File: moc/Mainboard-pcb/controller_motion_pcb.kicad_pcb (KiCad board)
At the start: 2 copper layers, 156 x 30 mm, 30 parts, among them J1 Conn_01x08_Female, J2 Conn_01x09_Male, J3 Conn_01x06_Female, SW1 Rotary_Encoder_Switch, U1 TPIC6C595-SOIC, U2 TPIC6C595-SOIC

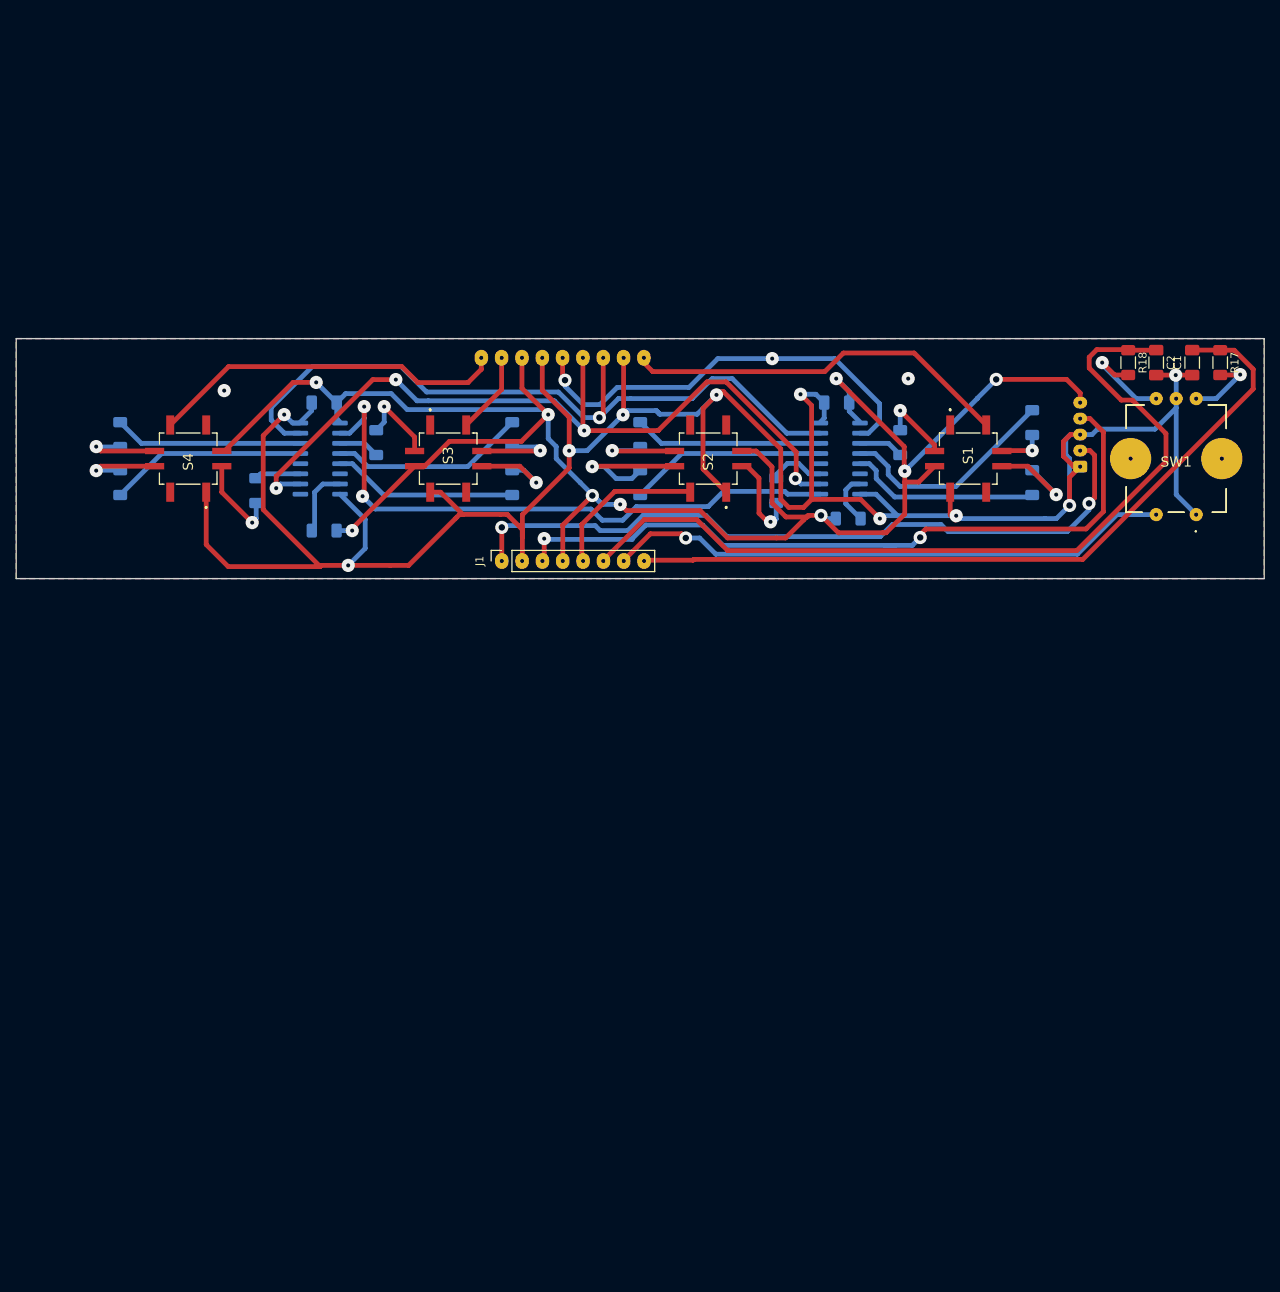
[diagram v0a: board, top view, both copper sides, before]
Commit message: hardware io funzt
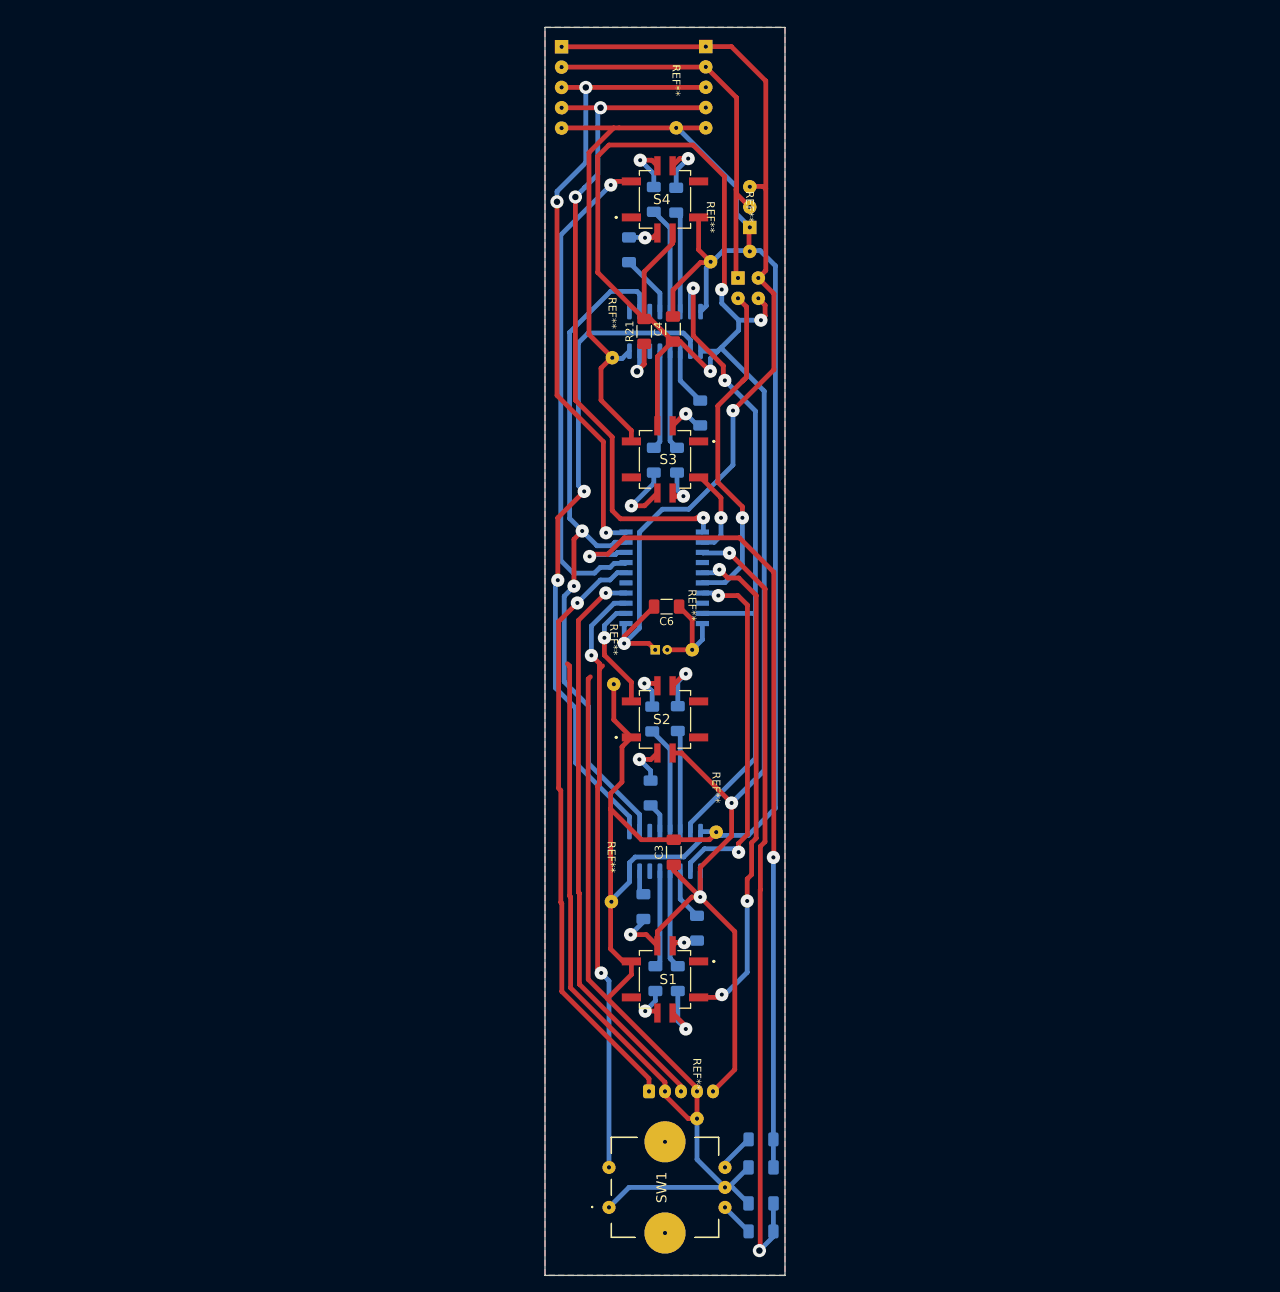
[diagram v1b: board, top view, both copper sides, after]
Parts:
- added C5: 10uF, Capacitor_THT:CP_Radial_D4.0mm_P1.50mm, B.Cu at (149.9, 101.5)
- added C6: 100nF, Capacitor_SMD:C_1206_3216Metric_Pad1.33x1.80mm_HandSolder, F.Cu at (151.3, 96.1)
- added J4: UPDI_Interface, Connector_PinHeader_2.54mm:PinHeader_1x03_P2.54mm_Vertical, B.Cu at (161.7, 48.7)
- added J5: Programm_Jumper, Connector_PinHeader_2.54mm:PinHeader_2x02_P2.54mm_Vertical, B.Cu at (160.2, 55.0)
- added REF**: thermal_via, .Ambisonic:thermal_via, F.Cu at (154.0, 95.9)
- added REF**: thermal_via, .Ambisonic:thermal_via, F.Cu at (154.6, 154.5)
- added REF**: thermal_via, .Ambisonic:thermal_via, F.Cu at (152.0, 30.3)
- added REF**: thermal_via, .Ambisonic:thermal_via, F.Cu at (157.0, 118.7)
- added REF**: thermal_via, .Ambisonic:thermal_via, F.Cu at (161.2, 46.1)
- added REF**: thermal_via, .Ambisonic:thermal_via, F.Cu at (144.2, 100.2)
- added REF**: thermal_via, .Ambisonic:thermal_via, F.Cu at (156.3, 47.4)
- added REF**: thermal_via, .Ambisonic:thermal_via, F.Cu at (143.9, 127.4)
- added REF**: thermal_via, .Ambisonic:thermal_via, F.Cu at (144.0, 59.4)
- added U3: ATtiny1626, .Ambisonic:attiny1626, B.Cu at (151.0, 92.5)
- C1, C2, R17, R18: moved to B.Cu
- C3, C4, R21: moved to F.Cu
- J1: value Conn_01x08_Female -> SPI_Female; footprint Connector_PinSocket_2.54mm:PinSocket_1x08_P2.54mm_Vertical -> Connector_PinSocket_2.54mm:PinSocket_1x05_P2.54mm_Horizontal; moved to B.Cu
- J2: value Conn_01x09_Male -> SPI_Male; footprint .Ambisonic:Header-01x09-p2.54-selfsolder -> Connector_PinHeader_2.54mm:PinHeader_1x05_P2.54mm_Horizontal
- moved R17 122.8 mm to (163.1, 174.2), turned to 180 degrees
- moved C1 118.1 mm to (163.1, 170.7), turned to 0 degrees
- moved SW1 114.8 mm to (151.1, 171.2), turned to 90 degrees
- moved C2 112.1 mm to (163.1, 166.2), turned to 180 degrees
- moved R18 107.4 mm to (163.1, 162.7), turned to 180 degrees
- moved J3 94.9 mm to (149.1, 156.7), turned to 0 degrees
- moved R5 82.4 mm to (152.7, 142.6)
- moved R6 77.9 mm to (149.9, 142.6), turned to 90 degrees
- moved R14 75.5 mm to (149.7, 45.2)
- moved R15 75.4 mm to (152.5, 45.3), turned to -90 degrees
- moved S1 75.3 mm to (151.1, 142.7), turned to 0 degrees
- moved J1 69.2 mm to (156.2, 26.1), turned to 180 degrees
- moved S4 67.8 mm to (151.1, 45.2), turned to 180 degrees
- moved R7 65.8 mm to (155.1, 136.3), turned to 90 degrees
- moved C3 59.8 mm to (152.2, 126.8), turned to 90 degrees
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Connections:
- net Net-(U1-Pad9) renamed PSHFDATA2
- J1 pad 1: ADC1 -> VCC_w
- J1 pad 2: GND -> UPDI_w
- J1 pad 3: ADC0 -> SDA
- J1 pad 4: VCC -> SCL
- J1 pad 5: BUT1 -> GND
- J2 pad 1: BUT0 -> VCC_w
- J2 pad 2: GND -> UPDI_w
- J2 pad 3: PSHFCLK -> SDA
- J2 pad 4: PSHFUDATE -> SCL
- J2 pad 5: PSHFDATA -> GND
- J3 pad 1: GND -> ADC1
- J3 pad 2: ADC1 -> GND
- J3 pad 3: GND -> ADC0
- J3 pad 4: ADC0 -> GND
- S4 pad 1: GND -> unconnected-(S4-Pad1)
- S4 pad 2: unconnected-(S4-Pad2) -> GND
- S4 pad 3: unconnected-(S4-Pad3) -> BUT3
- S4 pad 4: BUT3 -> unconnected-(S4-Pad4)
- U1 pad 11: S2_B -> unconnected-(U1-Pad11)
- U1 pad 12: unconnected-(U1-Pad12) -> S2_B
- U1 pad 15: PSHFCLK -> PSFHCLK
- U2 pad 11: S4_B -> unconnected-(U2-Pad11)
- U2 pad 12: unconnected-(U2-Pad12) -> S4_B
- U2 pad 15: PSHFCLK -> PSFHCLK
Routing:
- net GND: track 314.1 -> 442.3 mm, vias 12 -> 0
- net VCC_w: track 0.00 -> 123.6 mm, vias 0 -> 2
- net PSHFCLK: track 91.8 -> 0.00 mm, vias 1 -> 0
- net SCL: track 0.00 -> 85.3 mm, vias 0 -> 3
- net PSFHCLK: track 0.00 -> 84.5 mm, vias 0 -> 2
- net SDA: track 0.00 -> 80.3 mm, vias 0 -> 3
- net UPDI_w: track 0.00 -> 49.1 mm
- net UPDI: track 0.00 -> 42.9 mm, vias 0 -> 1
- net ADC0: track 91.8 -> 71.6 mm, vias 2 -> 1
- net BUT3: track 44.2 -> 61.6 mm, vias 0 -> 1
- net ADC1: track 91.0 -> 74.4 mm, vias 2 -> 1
- net S1_R: track 27.8 -> 12.3 mm
- net BUT0: track 47.9 -> 63.2 mm, vias 0 -> 3
- net PSHFUDATE: track 100.0 -> 87.5 mm, vias 4 -> 2
- net Net-(R8-Pad1): track 17.4 -> 5.05 mm
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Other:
- board size 156 x 30 mm -> 30 x 156 mm

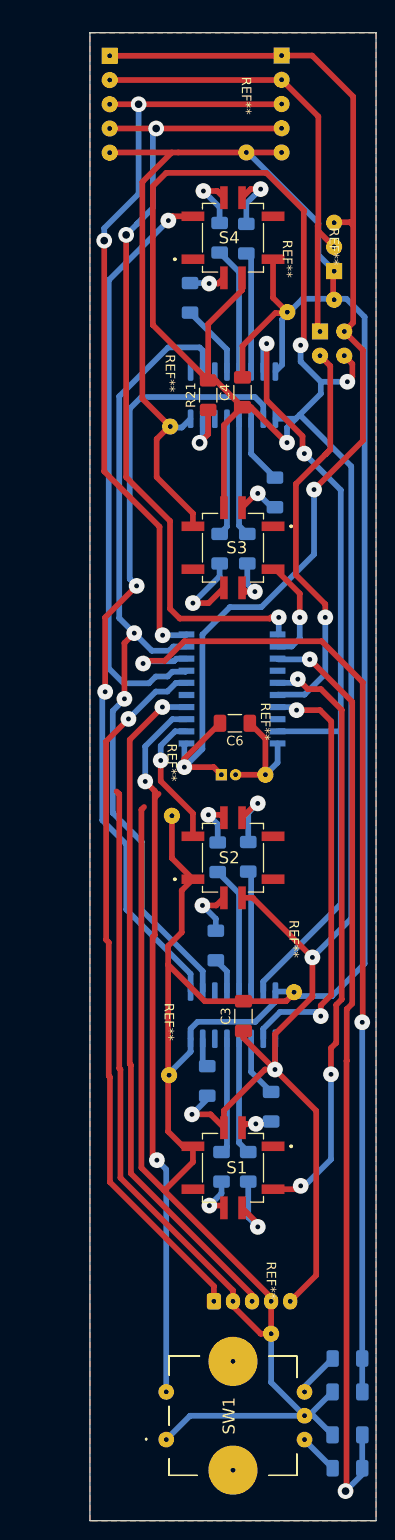
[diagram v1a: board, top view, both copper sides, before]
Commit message: clean up
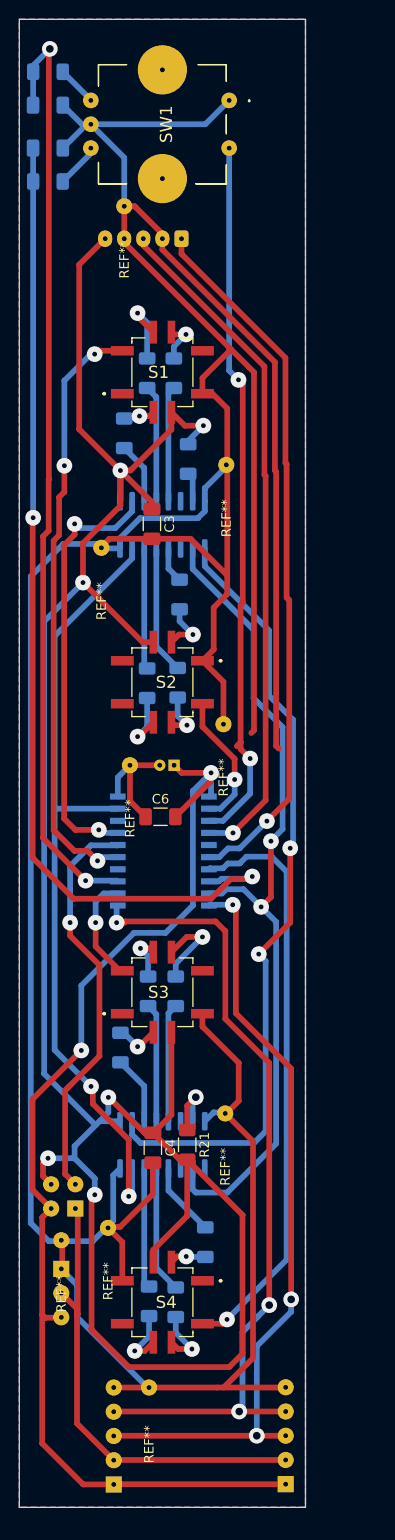
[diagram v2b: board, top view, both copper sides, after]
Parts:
- moved J2 150.9 mm to (156.6, 175.9), turned to 0 degrees
- moved J1 150.8 mm to (138.6, 175.9), turned to 0 degrees
- moved R17 149.7 mm to (131.7, 27.8), turned to 0 degrees
- moved C1 142.9 mm to (131.7, 31.3), turned to 180 degrees
- moved REF** 141.7 mm to (142.8, 171.7), turned to 90 degrees
- moved SW1 140.6 mm to (143.7, 30.8), turned to -90 degrees
- moved C2 134.1 mm to (131.7, 35.8), turned to 0 degrees
- moved R18 127.3 mm to (131.7, 39.3), turned to 0 degrees
- moved REF** 113.2 mm to (133.6, 155.9), turned to 90 degrees
- moved R15 111.9 mm to (142.3, 156.7), turned to 90 degrees
- moved S4 111.8 mm to (143.7, 156.8), turned to 0 degrees
- moved R14 111.7 mm to (145.1, 156.8), turned to 90 degrees
- moved J3 111.5 mm to (145.7, 45.3), turned to 180 degrees
- moved REF** 108.7 mm to (138.5, 154.6), turned to 90 degrees
- moved J4 108.4 mm to (133.1, 153.3), turned to 180 degrees
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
